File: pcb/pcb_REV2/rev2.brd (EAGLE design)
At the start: 95.2 x 80 mm, 73 parts, among them IC1 PIC24FJ128GA010, IC2 LM1117-XX, IC3 MAX6520, J1 RJ11-6X

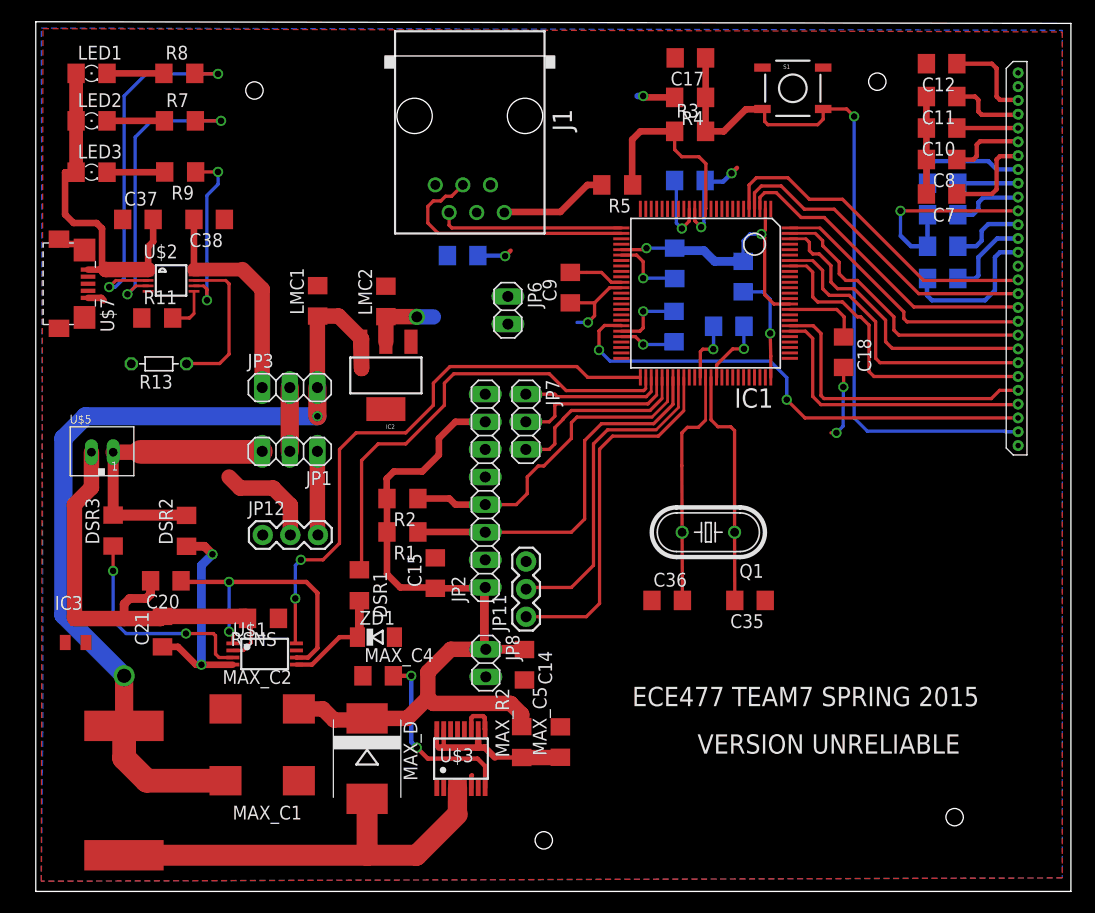
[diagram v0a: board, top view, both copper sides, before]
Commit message: latest
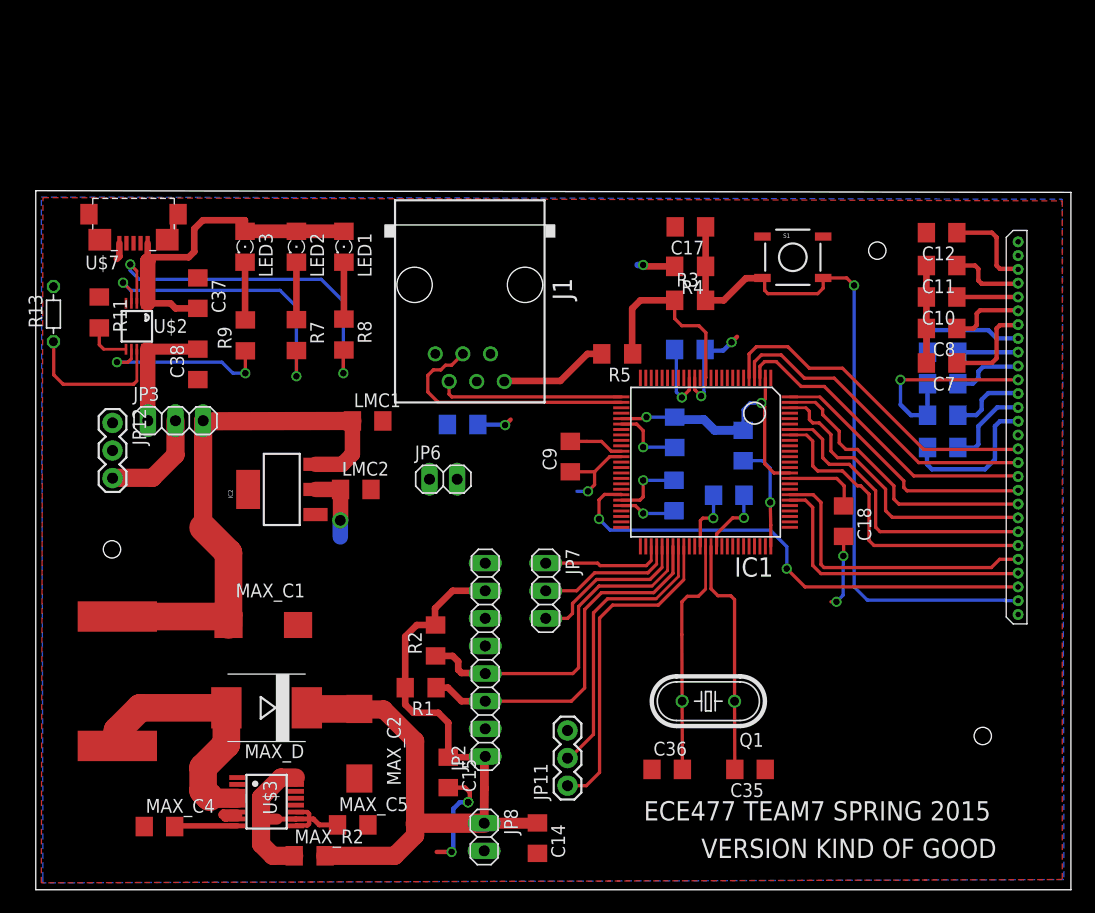
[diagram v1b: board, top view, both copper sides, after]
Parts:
- removed C20, C21: 0.1uF, rcl:C1206
- removed DSR1: 150, rcl:R1206
- removed DSR2: 500, rcl:R1206
- removed DSR3: 1K, rcl:R1206
- removed IC3: MAX6520, maxim:SOT23
- removed JP1: gauge_selector, pinhead:1X03
- removed RSNS: (no value), rcl:R1206
- removed U$1: DS2781E, fuelgauge:TSSOP8
- removed U$5: JST-PH_2-PIN_HEADER, SRG:JST_B2B-PH_HEADER
- removed ZD1: 5.6V, diode:SOD80C
- MAX_C1, MAX_C2: device adafruit:D/7343-31W -> rcl:CT7343
- moved R8 28.4 mm to (28.3, 51.1), turned to 270 degrees
- moved LED1 28.2 mm to (28.3, 59.2), turned to 270 degrees
- moved MAX_C4 24.4 mm to (11.4, 5.84)
- moved R7 22.4 mm to (24.0, 51.1), turned to 270 degrees
- moved MAX_R2 22.1 mm to (25.2, 3.15), turned to 0 degrees
- moved LED2 22.1 mm to (24.0, 59.2), turned to 270 degrees
- moved MAX_C5 20.6 mm to (29.2, 5.99), turned to 0 degrees
- moved C15 18.4 mm to (37.9, 10.8), turned to 270 degrees
- moved U$3 18.3 mm to (21.2, 8.13), turned to 270 degrees
- moved LMC2 17.5 mm to (29.4, 36.9), turned to 0 degrees
- moved JP12 17.2 mm to (7.06, 43.0), turned to 270 degrees
- moved JP6 16.6 mm to (37.5, 37.8), turned to 0 degrees
- moved R9 16.2 mm to (19.3, 51.0), turned to 90 degrees
- moved JP11 16.0 mm to (48.9, 9.60)
- moved JP8 16.0 mm to (41.2, 4.88)
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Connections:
- removed net BATT-: C20.2, C21.2, IC3.3, RSNS.2, U$1.2, U$5.P2
- removed net FG2_VCC: JP1.1, JP12.3
- removed net N$31: DSR1.2, U$1.5, ZD1.C
- removed net N$36: C21.1, DSR2.1, U$1.4
- removed net N$37: C20.1, U$1.1, U$1.6
- removed net N$39: DSR3.1, U$1.3
- removed net REAL_BATT+: DSR2.2, DSR3.2, JP1.3, U$5.P1
- net BATT+: now also JP12.3; no longer JP1.2
- net DS_DATA: no longer DSR1.1
- net GND: no longer IC3.1, IC3.2, RSNS.1, U$1.7, ZD1.A
- net PIO: no longer U$1.8
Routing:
- net PIO: track 53.2 -> 0.00 mm, vias 2 -> 0
- net DS_DATA: track 42.5 -> 0.00 mm
- net BATT-: track 41.9 -> 0.00 mm
- net AVIN: track 85.5 -> 50.6 mm, vias 2 -> 0
- net REAL_BATT+: track 26.3 -> 0.00 mm
- net N$37: track 26.2 -> 0.00 mm, vias 2 -> 0
- net N$36: track 20.4 -> 0.00 mm, vias 2 -> 0
- net N$39: track 20.3 -> 0.00 mm, vias 2 -> 0
- net N$35: track 41.1 -> 25.6 mm
- net N$40: track 17.5 -> 5.79 mm, vias 2 -> 0
- net N$31: track 10.1 -> 0.00 mm
- net N$51: track 21.3 -> 11.7 mm
- net FG2_VCC: track 7.70 -> 0.00 mm
- net N$38: track 16.7 -> 23.9 mm
- net GND: track 96.5 -> 101.3 mm, vias 9 -> 11
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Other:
- board size 95.2 x 80 mm -> 95.2 x 64.3 mm
- board text added: "VERSION KIND OF GOOD"
- board text removed: "VERSION UNRELIABLE"
